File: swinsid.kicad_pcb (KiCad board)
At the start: 2 copper layers, 17.5 x 36.6 mm, 14 parts, among them U1 ATmega88PA-AU, U2 SID6581, X1 SG-7050CAN

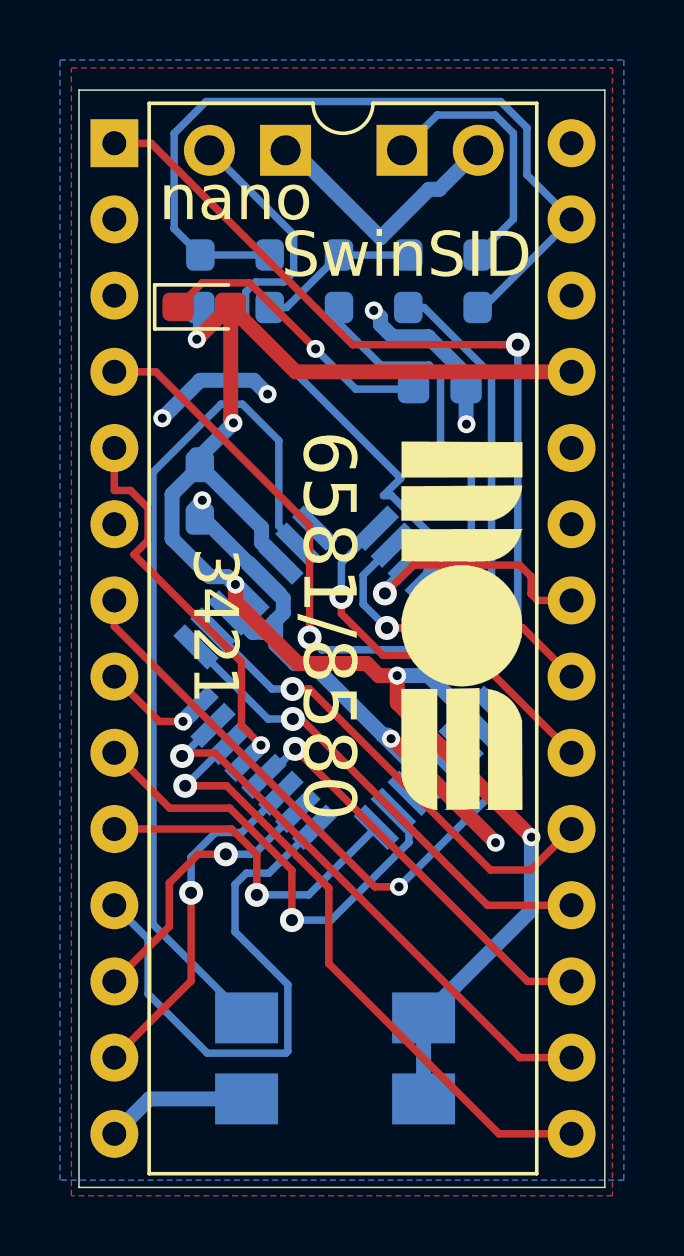
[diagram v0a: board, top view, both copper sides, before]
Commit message: Updated swinsid image
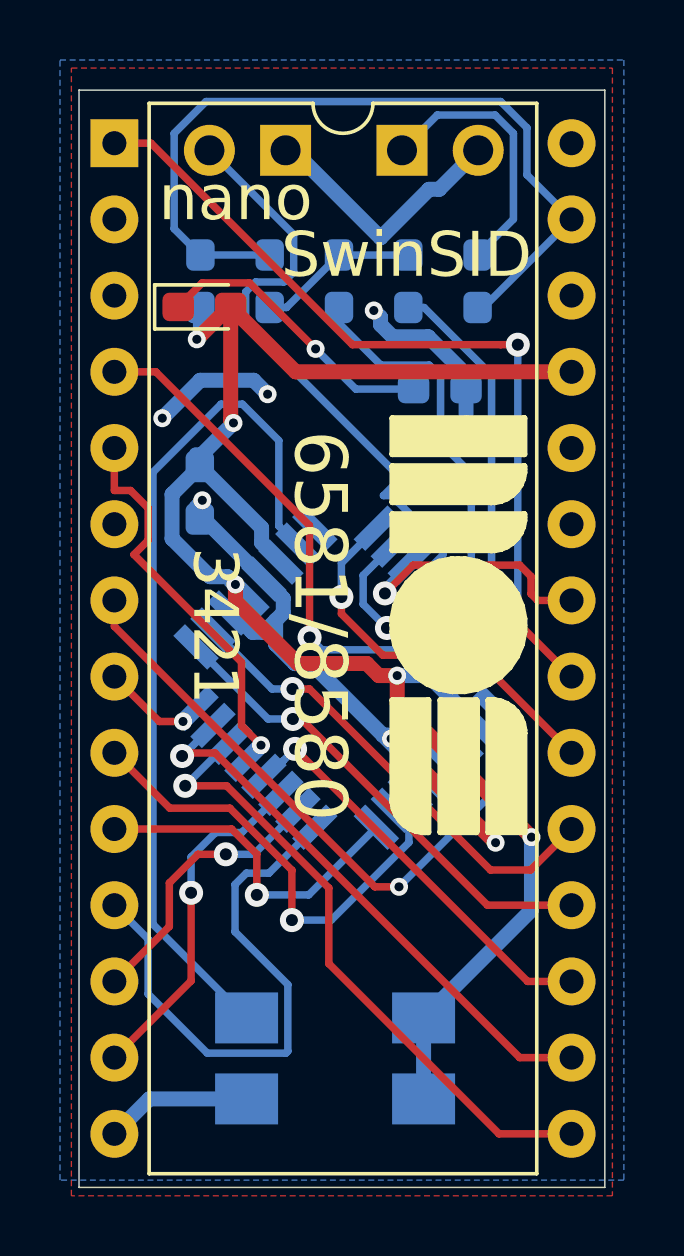
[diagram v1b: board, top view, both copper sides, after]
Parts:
- removed G***: LOGO, custom:mosBig
